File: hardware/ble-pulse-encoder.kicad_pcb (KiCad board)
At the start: 2 copper layers, 40 x 40 mm, 59 parts, among them J1 USB_B_Micro, J2 EZmate-3, J3 EZmate-4, J4 TC2030-IDC-NL, J5 EZmate-5, Q1 BSS84, Q2 Q_Photo_NPN_CBE, Q3 Q_Photo_NPN_CBE, SW1 SW_Push, SW2 SW_Push, U1 STBC08, U2 nRF52832-QFxx, U3 MIC5301, Y1 32.768kHz, Y2 32MHz

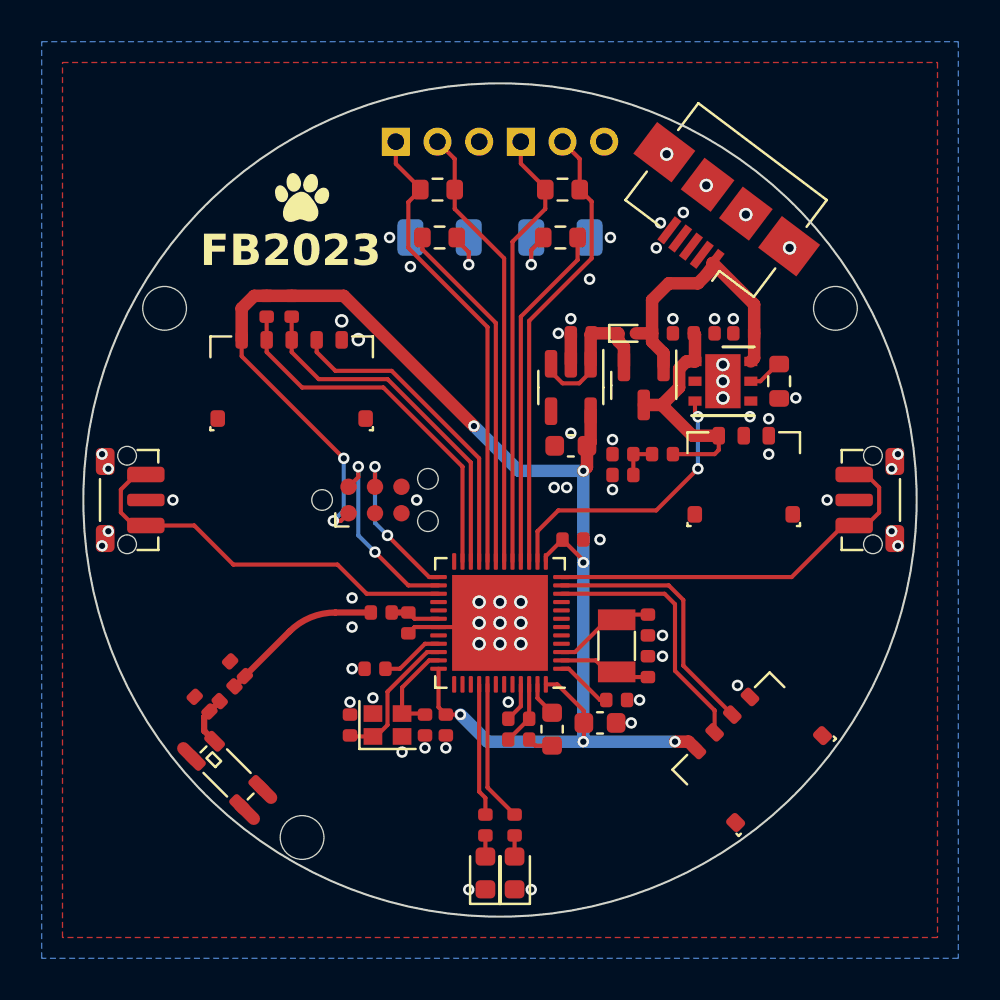
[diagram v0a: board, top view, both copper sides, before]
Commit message: r0
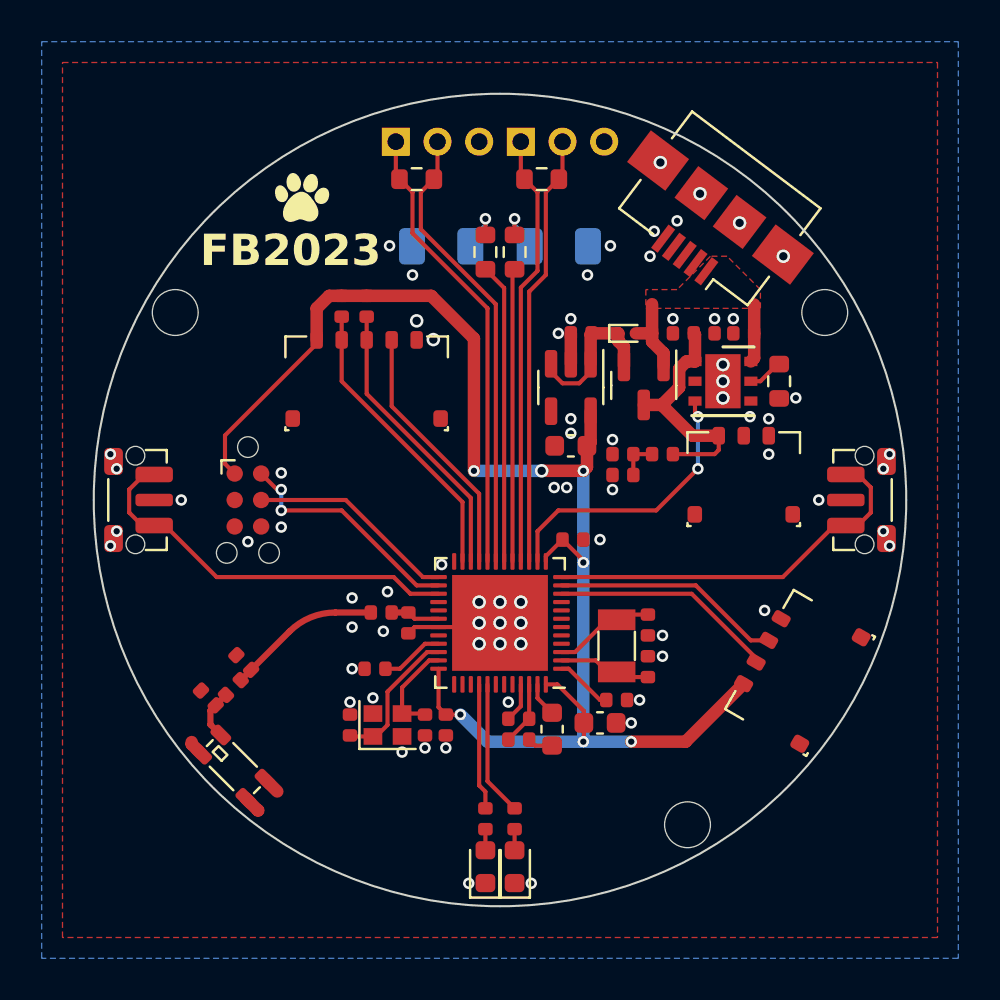
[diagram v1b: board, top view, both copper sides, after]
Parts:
- removed REF** (x3): MountingHole_2.1mm, MountingHole:MountingHole_2.1mm
- added H1: MountingHole_2.2mm_M2, MountingHole:MountingHole_2.2mm_M2, F.Cu at (133.4, 82.0)
- added H2: MountingHole_2.2mm_M2, MountingHole:MountingHole_2.2mm_M2, F.Cu at (164.6, 82.0)
- added H3: MountingHole_2.2mm_M2, MountingHole:MountingHole_2.2mm_M2, F.Cu at (158.0, 106.6)
- moved J4 6.10 mm to (136.9, 91.0), turned to -90 degrees
- moved J3 4.48 mm to (163.4, 99.3), turned to 60 degrees
- moved J5 3.60 mm to (142.6, 85.4)
- moved R7 3.60 mm to (142.6, 81.7)
- moved R8 3.60 mm to (141.4, 81.7)
- moved R10 2.31 mm to (149.7, 79.1), turned to 90 degrees
- moved R9 2.31 mm to (148.3, 79.1), turned to 90 degrees
- moved R11 1.12 mm to (151.0, 75.6)
- moved R12 1.12 mm to (145.0, 75.6)
- moved J1 0.50 mm to (158.8, 78.0)
- moved D4 0.43 mm to (146.2, 78.8)
- moved D5 0.43 mm to (151.8, 78.8)
- moved C16 0.42 mm to (135.0, 100.5)
- moved AE1 0.42 mm to (136.2, 103.8)
- moved C14 0.42 mm to (136.7, 98.8)
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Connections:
- U2 pad 16: /D0_PWR -> /PH0_SENSE
- U2 pad 17: /PH0_SENSE -> /D0_PWR
- U2 pad 18: /PH1_PWR -> /D1_PWR
- U2 pad 19: /D1_PWR -> /PH1_PWR
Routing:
- net +5V: track 13.6 -> 6.77 mm
- net /SCL: track 17.9 -> 14.2 mm
- net /SDA: track 17.2 -> 13.8 mm
- net /EXT_IRQ: track 15.4 -> 12.4 mm
- net /D1_PWR: track 17.0 -> 14.4 mm
- net /D0_PWR: track 16.7 -> 14.1 mm
- net /NRF_SWCLK: track 7.79 -> 10.0 mm, vias 2 -> 0
- net /NRF_SWDIO: track 9.31 -> 11.3 mm
- net /UART_RX: track 12.6 -> 10.8 mm
- net /UART_TX: track 12.6 -> 11.0 mm
- net /PH0_PWR: track 22.0 -> 20.8 mm
- net GND: track 10.8 -> 10.7 mm, vias 67 -> 73
- net +3V3: vias 8 -> 7
- added copper zone on F.Cu, net +5V
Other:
- board size 40 x 40 mm -> 39 x 39 mm
- board text added: "Photo: 100 cuts, 3.6 per cut, 7*.9 + 2 half cuts 90+(360/100*7.25)/2 = 103.05 90-(360/100*7.25)/2 = 76.95 R12.5"
